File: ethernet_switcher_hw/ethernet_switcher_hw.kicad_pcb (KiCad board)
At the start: 2 copper layers, 103 parts, among them Q1 BSS138, Q10 BSS138, Q11 BSS138, Q12 BSS138, Q13 BSS138, Q14 BSS138, Q15 BSS138, Q16 BSS138, Q17 BSS138, Q18 BSS138, Q19 BSS138, Q2 BSS138, Q20 BSS138, Q3 BSS138, Q4 BSS138, Q5 BSS138, Q6 BSS138, Q7 BSS138, Q8 BSS138, Q9 BSS138, X1 Screw_Terminal_01x02

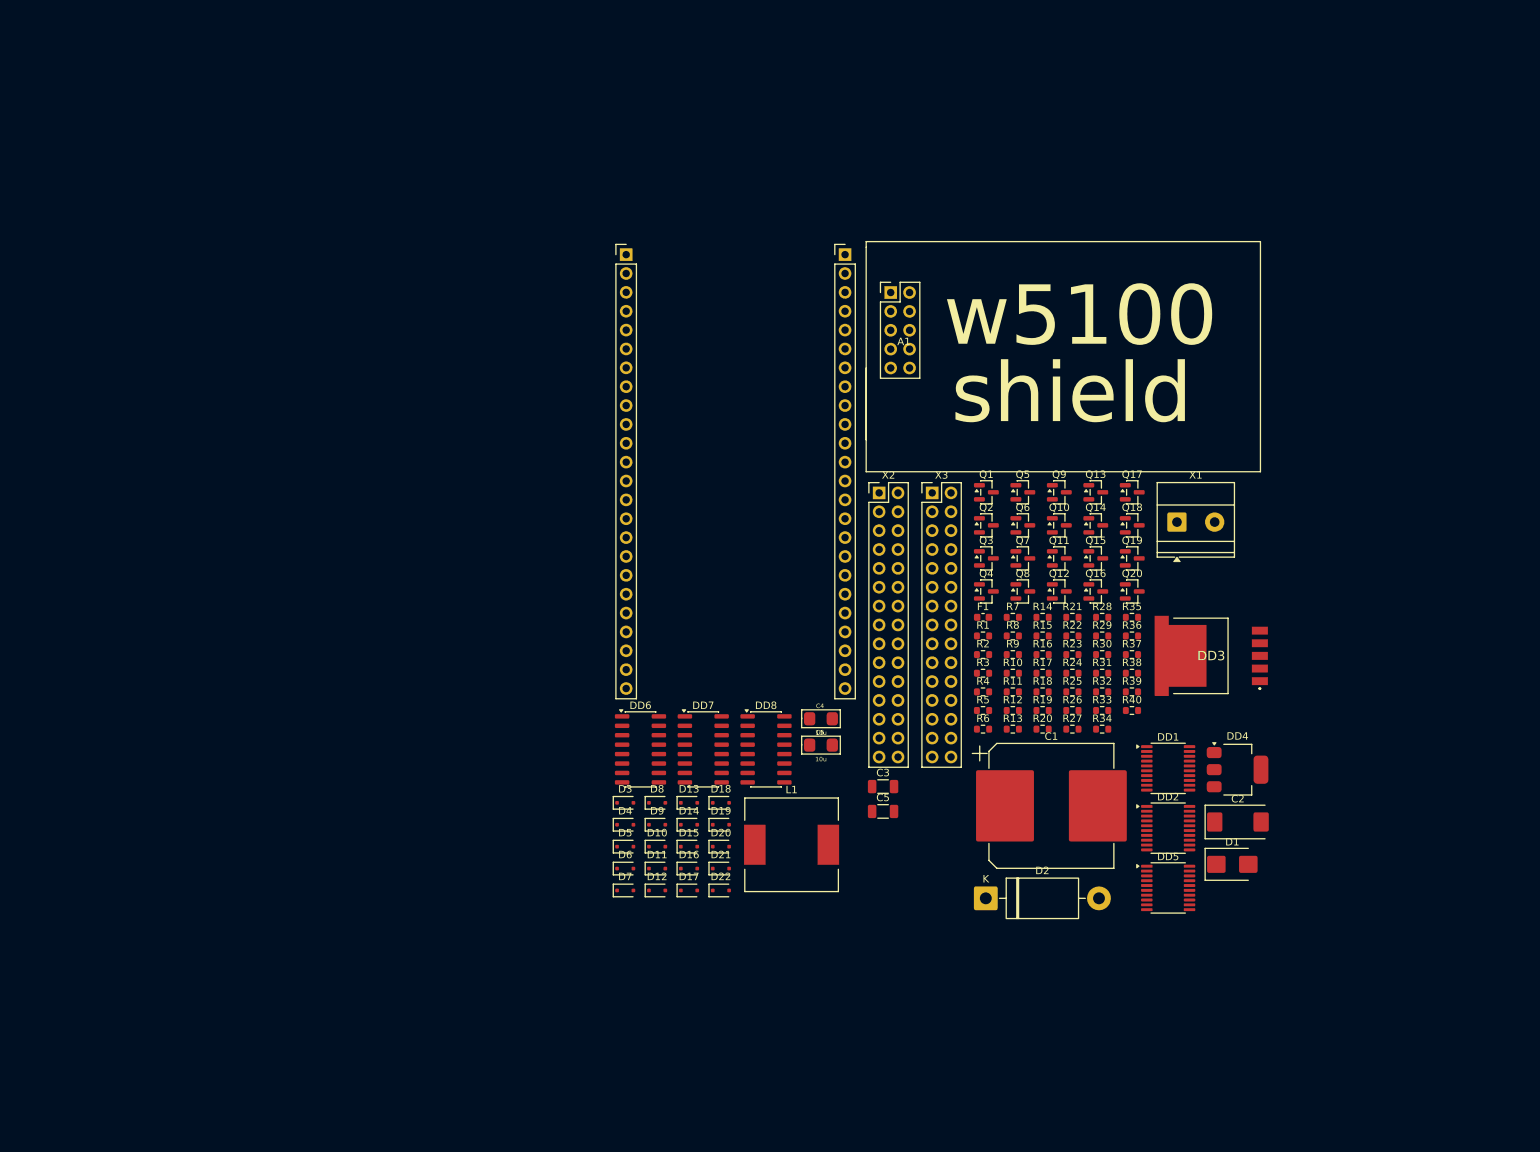
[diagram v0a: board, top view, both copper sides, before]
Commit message: ready project
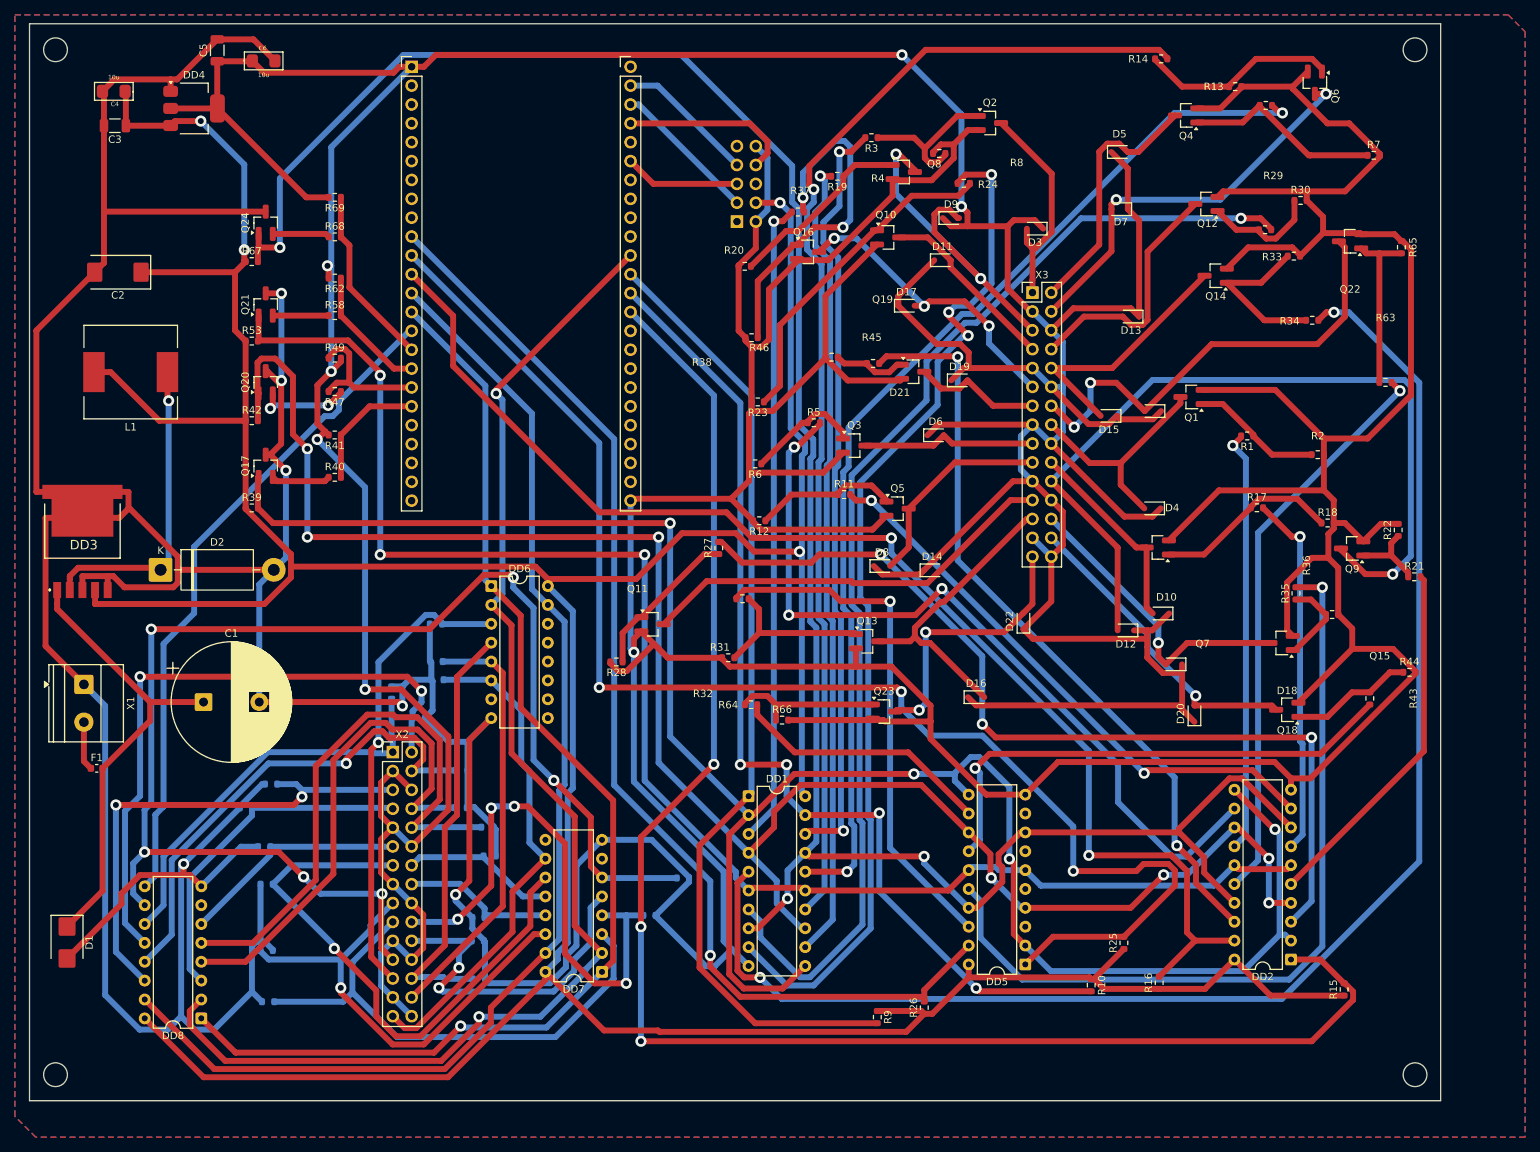
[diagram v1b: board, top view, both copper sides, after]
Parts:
- added G***: LOGO, LOGO, B.Cu at (41.0, 46.3)
- added H1: MountingHole_3.2mm_M3, MountingHole:MountingHole_3.2mm_M3, F.Cu at (203.6, 159.3)
- added H2: MountingHole_3.2mm_M3, MountingHole:MountingHole_3.2mm_M3, F.Cu at (20.5, 159.3)
- added H3: MountingHole_3.2mm_M3, MountingHole:MountingHole_3.2mm_M3, F.Cu at (20.5, 21.3)
- added H4: MountingHole_3.2mm_M3, MountingHole:MountingHole_3.2mm_M3, F.Cu at (203.6, 21.3)
- added Q21: NPN, Package_TO_SOT_SMD:SOT-23_Handsoldering, F.Cu at (48.8, 55.6)
- added Q22: AO3422A, Package_TO_SOT_SMD:SOT-23_Handsoldering, F.Cu at (194.8, 47.1)
- added Q23: AO3422A, Package_TO_SOT_SMD:SOT-23_Handsoldering, F.Cu at (132.1, 110.4)
- added Q24: NPN, Package_TO_SOT_SMD:SOT-23_Handsoldering, F.Cu at (48.8, 44.6)
- added R41: 20k, Resistor_SMD:R_0603_1608Metric, F.Cu at (58.1, 73.2)
- added R42: 4.7k, Resistor_SMD:R_0603_1608Metric, F.Cu at (46.9, 71.3)
- added R43: 100, Resistor_SMD:R_0603_1608Metric, F.Cu at (197.5, 108.7)
- added R44: 100k, Resistor_SMD:R_0603_1608Metric, F.Cu at (202.8, 105.1)
- added R45: 100, Resistor_SMD:R_0603_1608Metric, F.Cu at (130.6, 63.6)
- added R46: 100k, Resistor_SMD:R_0603_1608Metric, F.Cu at (125.0, 62.7)
- added R47: 1k, Resistor_SMD:R_0603_1608Metric, F.Cu at (58.1, 67.3)
- added R48: 100k, Resistor_SMD:R_0603_1608Metric, B.Cu at (49.5, 120.2)
- added R49: 20k, Resistor_SMD:R_0603_1608Metric, F.Cu at (58.1, 62.8)
- added R50: 100k, Resistor_SMD:R_0603_1608Metric, B.Cu at (77.3, 141.3)
- added R51: 100k, Resistor_SMD:R_0603_1608Metric, B.Cu at (75.2, 118.3)
- added R52: 100k, Resistor_SMD:R_0603_1608Metric, B.Cu at (100.5, 137.9)
- added R53: 4.7k, Resistor_SMD:R_0603_1608Metric, F.Cu at (46.9, 60.5)
- added R54: 100k, Resistor_SMD:R_0603_1608Metric, B.Cu at (69.4, 111.3)
- added R55: 100k, Resistor_SMD:R_0603_1608Metric, B.Cu at (49.1, 149.5)
- added R56: 100k, Resistor_SMD:R_0603_1608Metric, B.Cu at (48.9, 142.6)
- added R57: 100k, Resistor_SMD:R_0603_1608Metric, B.Cu at (65.8, 107.9)
- added R58: 1k, Resistor_SMD:R_0603_1608Metric, F.Cu at (58.1, 57.1)
- added R59: 100k, Resistor_SMD:R_0603_1608Metric, B.Cu at (77.5, 138.2)
- added R60: 100k, Resistor_SMD:R_0603_1608Metric, B.Cu at (79.0, 129.9)
- added R61: 100k, Resistor_SMD:R_0603_1608Metric, B.Cu at (48.9, 133.7)
- added R62: 20k, Resistor_SMD:R_0603_1608Metric, F.Cu at (58.1, 52.1)
- added R63: 100, Resistor_SMD:R_0603_1608Metric, F.Cu at (199.6, 66.1)
- added R64: 100, Resistor_SMD:R_0603_1608Metric, F.Cu at (114.2, 109.5)
- added R65: 100k, Resistor_SMD:R_0603_1608Metric, F.Cu at (201.7, 47.9)
- added R66: 100k, Resistor_SMD:R_0603_1608Metric, F.Cu at (118.3, 111.6)
- added R67: 4.7k, Resistor_SMD:R_0603_1608Metric, F.Cu at (46.9, 49.8)
- added R68: 1k, Resistor_SMD:R_0603_1608Metric, F.Cu at (58.1, 46.5)
- added R69: 20k, Resistor_SMD:R_0603_1608Metric, F.Cu at (58.1, 41.2)
- added R70: 100k, Resistor_SMD:R_0603_1608Metric, B.Cu at (105.0, 132.8)
- added R71: 100k, Resistor_SMD:R_0603_1608Metric, B.Cu at (46.1, 123.4)
- added R72: 100k, Resistor_SMD:R_0603_1608Metric, B.Cu at (71.7, 98.7)
- added R73: 100k, Resistor_SMD:R_0603_1608Metric, B.Cu at (75.0, 123.4)
- added R74: 100k, Resistor_SMD:R_0603_1608Metric, B.Cu at (77.5, 146.4)
- added R75: 100k, Resistor_SMD:R_0603_1608Metric, B.Cu at (78.7, 126.0)
- added R76: 100k, Resistor_SMD:R_0603_1608Metric, B.Cu at (71.8, 103.7)
- added R77: 100k, Resistor_SMD:R_0603_1608Metric, B.Cu at (48.6, 128.6)
- added R78: 100k, Resistor_SMD:R_0603_1608Metric, B.Cu at (71.9, 106.2)
- A1: moved to B.Cu
- C1: footprint Capacitor_SMD:CP_Elec_16x22 -> Capacitor_THT:CP_Radial_D16.0mm_P7.50mm
- DD1, DD2, DD5: footprint Package_SO:SSOP-20_4.4x6.5mm_P0.65mm -> Package_DIP:DIP-20_W7.62mm
- DD6, DD7, DD8: footprint Package_SO:SOIC-16_3.9x9.9mm_P1.27mm -> Package_DIP:DIP-16_W7.62mm
- Q1, Q10, Q11, Q12, Q13, Q14, Q15, Q16, Q18, Q19, Q2, Q3, Q4, Q5, Q6, Q7, Q8, Q9: value BSS138 -> AO3422A; footprint Package_TO_SOT_SMD:SOT-23 -> Package_TO_SOT_SMD:SOT-23_Handsoldering
- Q17, Q20: value BSS138 -> NPN; footprint Package_TO_SOT_SMD:SOT-23 -> Package_TO_SOT_SMD:SOT-23_Handsoldering
- R1, R17, R21, R29, R3, R31, R35, R37, R5, R8: value 10k -> 100
- R10, R16, R26: value 100k -> 20k
- R11, R14, R19, R24, R27, R34: value 100k -> 100
- R12, R13, R20, R23, R28, R33, R38: value 10k -> 100k
- R15, R25, R9: value 10k -> 20k
- R39: value 100k -> 4.7k
- R40: value 100k -> 1k
- moved C2 168.0 mm to (28.9, 51.3), turned to 180 degrees
- moved DD4 166.3 mm to (39.1, 29.2)
- moved D1 157.3 mm to (22.1, 141.5), turned to -90 degrees
- moved DD3 152.8 mm to (24.1, 87.5), turned to -90 degrees
- moved X1 148.8 mm to (24.3, 106.8), turned to -90 degrees
- moved C3 136.4 mm to (28.5, 31.6), turned to 180 degrees
- moved C5 136.2 mm to (42.3, 21.4), turned to 90 degrees
- moved C4 127.3 mm to (28.3, 26.9), turned to 180 degrees
- moved R39 121.1 mm to (46.9, 83.0)
- moved F1 121.1 mm to (26.0, 118.1)
- moved Q20 120.0 mm to (48.8, 66.1), turned to 90 degrees
- moved D2 119.6 mm to (34.6, 91.3)
- moved C6 118.8 mm to (48.5, 22.8)
- moved Q17 116.7 mm to (48.8, 77.3), turned to 90 degrees
- moved C1 115.0 mm to (40.4, 109.2)
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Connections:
- D10 pad 1: Net-(D10-K) -> +3.3V
- D10 pad 2: /r6p1 -> /r6p2
- D11 pad 1: Net-(D11-K) -> +3.3V
- D11 pad 2: /r2p0 -> /r2p1
- D12 pad 1: Net-(D12-K) -> +3.3V
- D12 pad 2: /r7p0 -> /r7p1
- D13 pad 1: Net-(D11-K) -> +3.3V
- D13 pad 2: /r2p1 -> /r2p2
- D14 pad 1: Net-(D12-K) -> +3.3V
- D14 pad 2: /r7p1 -> /r7p2
- D15 pad 1: Net-(D15-K) -> +3.3V
- D15 pad 2: /r3p0 -> /r3p1
- D16 pad 1: Net-(D16-K) -> +3.3V
- D16 pad 2: /r8p0 -> /r8p1
- D17 pad 1: Net-(D15-K) -> +3.3V
- D17 pad 2: /r3p1 -> /r3p2
- D18 pad 1: Net-(D16-K) -> +3.3V
- D18 pad 2: /r8p1 -> /r8p2
- D19 pad 1: Net-(D19-K) -> +3.3V
- D19 pad 2: /r4p0 -> /r4p1
- D20 pad 1: Net-(D20-K) -> +3.3V
- D20 pad 2: /r9p0 -> /r9p1
- D21 pad 1: Net-(D19-K) -> +3.3V
- D21 pad 2: /r4p1 -> /r4p2
- D22 pad 1: Net-(D20-K) -> +3.3V
- D22 pad 2: /r9p1 -> /r9p2
- D3 pad 1: Net-(D3-K) -> +3.3V
- D3 pad 2: /r0p0 -> /r0p1
- D4 pad 1: Net-(D4-K) -> +3.3V
- D4 pad 2: /r5p0 -> /r5p1
- D5 pad 1: Net-(D3-K) -> +3.3V
- D5 pad 2: /r0p1 -> /r0p2
- D6 pad 1: Net-(D4-K) -> +3.3V
- D6 pad 2: /r5p1 -> /r5p2
- D7 pad 1: Net-(D7-K) -> +3.3V
- D7 pad 2: /r1p0 -> /r1p1
- D8 pad 1: Net-(D10-K) -> +3.3V
- D8 pad 2: /r6p0 -> /r6p1
- D9 pad 1: Net-(D7-K) -> +3.3V
- D9 pad 2: /r1p1 -> /r1p2
- DD1 pad 11: /GPIO1_0 -> /line0_ctrl
- DD1 pad 13: /GPIO1_1 -> /line1_ctrl
- DD1 pad 15: /GPIO1_2 -> /line2_ctrl
- DD1 pad 17: /GPIO1_3 -> /line3_ctrl
- DD1 pad 2: /GPIO1_0 -> /line0_ctrl
- DD1 pad 20: +3.3V -> +5V
- DD1 pad 4: /GPIO1_1 -> /line1_ctrl
- DD1 pad 6: /GPIO1_2 -> /line2_ctrl
- DD1 pad 8: /GPIO1_3 -> /line3_ctrl
- DD2 pad 11: /GPIO1_0 -> /line0_ctrl
- DD2 pad 13: /GPIO1_1 -> /line1_ctrl
- DD2 pad 15: /GPIO1_2 -> /line2_ctrl
- DD2 pad 17: /GPIO1_3 -> /line3_ctrl
- DD2 pad 2: /GPIO1_0 -> /line0_ctrl
- DD2 pad 20: +3.3V -> +5V
- DD2 pad 4: /GPIO1_1 -> /line1_ctrl
- DD2 pad 6: /GPIO1_2 -> /line2_ctrl
- DD2 pad 8: /GPIO1_3 -> /line3_ctrl
- DD5 pad 11: /GPIO1_0 -> /line0_ctrl
- DD5 pad 13: /GPIO1_1 -> /line1_ctrl
- DD5 pad 15: /GPIO1_2 -> /line2_ctrl
- DD5 pad 17: /GPIO1_3 -> /line3_ctrl
- DD5 pad 2: /GPIO1_0 -> /line0_ctrl
- DD5 pad 20: +3.3V -> +5V
- DD5 pad 4: /GPIO1_1 -> /line1_ctrl
- DD5 pad 6: /GPIO1_2 -> /line2_ctrl
- DD5 pad 8: /GPIO1_3 -> /line3_ctrl
- Q17 pad 1: Net-(Q17-G) -> /line0_ctrl
- Q17 pad 2: GND -> Net-(Q17-B)
- Q17 pad 3: /r9p1 -> GND
- Q18 pad 3: /r4p1 -> /r9p1
- Q19 pad 3: /r4p2 -> /r4p1
- Q20 pad 1: Net-(Q20-G) -> /line1_ctrl
- Q20 pad 2: GND -> Net-(Q20-B)
- Q20 pad 3: /r9p2 -> GND
- R10 pad 1: Net-(Q5-G) -> +5V
- R10 pad 2: GND -> /GPIO0_9
- R11 pad 1: Net-(Q6-G) -> Net-(Q5-G)
- R11 pad 2: GND -> /r6p1_ctrl
- R12 pad 1: Net-(Q6-G) -> Net-(Q5-G)
- R12 pad 2: /r1p1_ctrl -> GND
- R13 pad 1: Net-(Q7-G) -> Net-(Q6-G)
- R13 pad 2: /r6p2_ctrl -> GND
- R14 pad 1: Net-(Q7-G) -> Net-(Q6-G)
- R14 pad 2: GND -> /r1p1_ctrl
- R15 pad 1: Net-(Q8-G) -> +5V
- R15 pad 2: /r1p2_ctrl -> /GPIO0_10
- R16 pad 1: Net-(Q8-G) -> +5V
- R16 pad 2: GND -> /GPIO1_7
- R17 pad 1: Net-(Q9-G) -> Net-(Q7-G)
- R17 pad 2: /r7p1_ctrl -> /r6p2_ctrl
- R18 pad 1: Net-(Q9-G) -> Net-(Q7-G)
- R19 pad 1: Net-(Q10-G) -> Net-(Q8-G)
- R19 pad 2: GND -> /r1p2_ctrl
- R20 pad 1: Net-(Q10-G) -> Net-(Q8-G)
- R20 pad 2: /r2p1_ctrl -> GND
- R21 pad 1: Net-(Q11-G) -> Net-(Q9-G)
- R21 pad 2: /r7p2_ctrl -> /r7p1_ctrl
- R22 pad 1: Net-(Q11-G) -> Net-(Q9-G)
- R23 pad 1: Net-(Q12-G) -> Net-(Q10-G)
- R23 pad 2: /r2p2_ctrl -> GND
- R24 pad 1: Net-(Q12-G) -> Net-(Q10-G)
- R24 pad 2: GND -> /r2p1_ctrl
- R25 pad 1: Net-(Q13-G) -> +5V
- R25 pad 2: /r8p1_ctrl -> /GPIO1_8
- R26 pad 1: Net-(Q13-G) -> +5V
- R26 pad 2: GND -> /GPIO1_9
- R27 pad 1: Net-(Q14-G) -> Net-(Q11-G)
- R27 pad 2: GND -> /r7p2_ctrl
- R28 pad 1: Net-(Q14-G) -> Net-(Q11-G)
- R28 pad 2: /r3p1_ctrl -> GND
- R29 pad 1: Net-(Q15-G) -> Net-(Q12-G)
- R29 pad 2: /r8p2_ctrl -> /r2p2_ctrl
- R30 pad 1: Net-(Q15-G) -> Net-(Q12-G)
- R31 pad 1: Net-(Q16-G) -> Net-(Q13-G)
- R31 pad 2: /r3p2_ctrl -> /r8p1_ctrl
- R32 pad 1: Net-(Q16-G) -> Net-(Q13-G)
- R33 pad 1: Net-(Q17-G) -> Net-(Q14-G)
- R33 pad 2: /r9p1_ctrl -> GND
- R34 pad 1: Net-(Q17-G) -> Net-(Q14-G)
- R34 pad 2: GND -> /r3p1_ctrl
- R35 pad 1: Net-(Q18-G) -> Net-(Q15-G)
- R35 pad 2: /r4p1_ctrl -> /r8p2_ctrl
- R36 pad 1: Net-(Q18-G) -> Net-(Q15-G)
- R37 pad 1: Net-(Q19-G) -> Net-(Q16-G)
- R37 pad 2: /r4p2_ctrl -> /r3p2_ctrl
- R38 pad 1: Net-(Q20-G) -> Net-(Q16-G)
- R38 pad 2: /r9p2_ctrl -> GND
- R39 pad 1: Net-(Q19-G) -> +5V
- R39 pad 2: GND -> /line0_ctrl
- R40 pad 1: Net-(Q20-G) -> Net-(Q17-B)
- R40 pad 2: GND -> /GPIO1_0
- R9 pad 1: Net-(Q5-G) -> +5V
- R9 pad 2: /r6p1_ctrl -> /GPIO0_8
- X2 pad 10: /r4t1 -> /r3t0
- X2 pad 11: /r5t0 -> /r3t1
- X2 pad 13: /r6t0 -> /r4t0
- X2 pad 14: /r6t1 -> /r4t1
- X2 pad 16: (no net) -> /r5t0
- X2 pad 17: (no net) -> /r5t1
- X2 pad 19: (no net) -> /r6t0
- X2 pad 20: (no net) -> /r6t1
- X2 pad 28: (no net) -> /r9t0
- X2 pad 29: (no net) -> /r9t1
- X2 pad 4: /r1t1 -> /r1t0
- X2 pad 5: /r2t0 -> /r1t1
- X2 pad 7: /r3t0 -> /r2t0
- X2 pad 8: /r3t1 -> /r2t1
- X3 pad 1: /r0p0 -> /r0p1
- X3 pad 10: /r4p1 -> /r3p1
- X3 pad 11: /r5p0 -> /r3p2
- X3 pad 12: /r5p1 -> +3.3V
- X3 pad 13: /r6p0 -> /r4p1
- X3 pad 14: /r6p1 -> /r4p2
- X3 pad 15: Net-(D19-K) -> +3.3V
- X3 pad 16: (no net) -> /r5p1
- X3 pad 17: (no net) -> /r5p2
- X3 pad 18: Net-(D4-K) -> +3.3V
- X3 pad 19: (no net) -> /r6p1
- X3 pad 2: /r0p1 -> /r0p2
- X3 pad 20: (no net) -> /r6p2
- X3 pad 21: Net-(D10-K) -> +3.3V
- X3 pad 22: /r7p0 -> /r7p1
- X3 pad 23: /r7p1 -> /r7p2
- X3 pad 24: Net-(D12-K) -> +3.3V
- X3 pad 25: /r8p0 -> /r8p1
- X3 pad 26: /r8p1 -> /r8p2
- X3 pad 27: /r9p1 -> +3.3V
- X3 pad 28: (no net) -> /r9p1
- X3 pad 29: (no net) -> /r9p2
- X3 pad 3: /r1p0 -> +3.3V
- X3 pad 30: Net-(D20-K) -> +3.3V
- X3 pad 5: /r2p0 -> /r1p2
- X3 pad 6: /r2p1 -> +3.3V
- X3 pad 7: /r3p0 -> /r2p1
- X3 pad 8: /r3p1 -> /r2p2
- X3 pad 9: /r4p0 -> +3.3V
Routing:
- net GND: track 0.00 -> 1277.5 mm, vias 0 -> 7
- net +3.3V: track 0.00 -> 648.2 mm, vias 0 -> 6
- net +5V: track 0.00 -> 557.9 mm, vias 0 -> 4
- net /line3_ctrl: track 0.00 -> 301.5 mm, vias 0 -> 3
- net /line0_ctrl: track 0.00 -> 266.6 mm, vias 0 -> 4
- net /line1_ctrl: track 0.00 -> 243.7 mm, vias 0 -> 7
- net /GPIO0_10: track 0.00 -> 216.4 mm, vias 0 -> 3
- net /line2_ctrl: track 0.00 -> 210.0 mm, vias 0 -> 3
- net /r3p1_ctrl: track 0.00 -> 197.4 mm, vias 0 -> 2
- net /r7t1: track 0.00 -> 190.1 mm, vias 0 -> 6
- net /GPIO1_8: track 0.00 -> 188.5 mm, vias 0 -> 3
- net /GPIO0_7: track 0.00 -> 176.9 mm, vias 0 -> 2
- net /GPIO1_7: track 0.00 -> 173.1 mm, vias 0 -> 2
- net /GPIO1_6: track 0.00 -> 164.0 mm
- net /GPIO1_5: track 0.00 -> 161.2 mm, vias 0 -> 1
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- added copper zone on B.Cu, net GND
- added copper zone on F.Cu, net GND
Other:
- board outline added: 190 x 145 mm
